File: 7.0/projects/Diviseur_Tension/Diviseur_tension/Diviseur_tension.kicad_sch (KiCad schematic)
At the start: 6 parts, among them Q1 2N2219

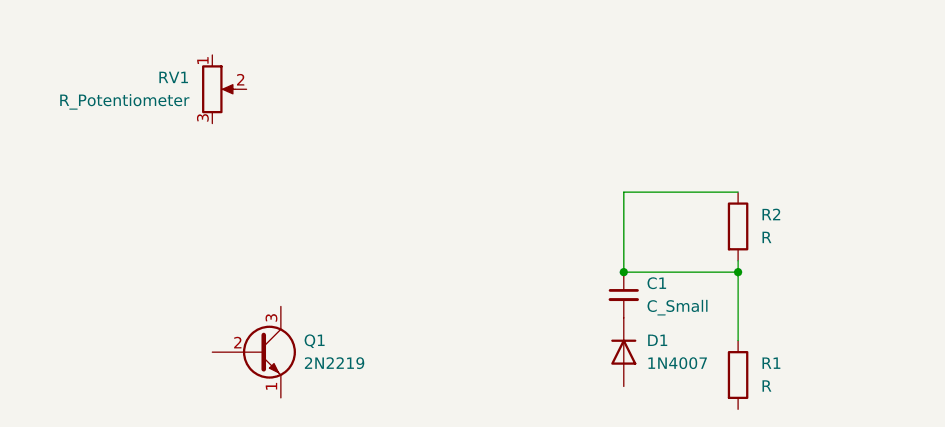
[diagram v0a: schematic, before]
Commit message: new modifcation
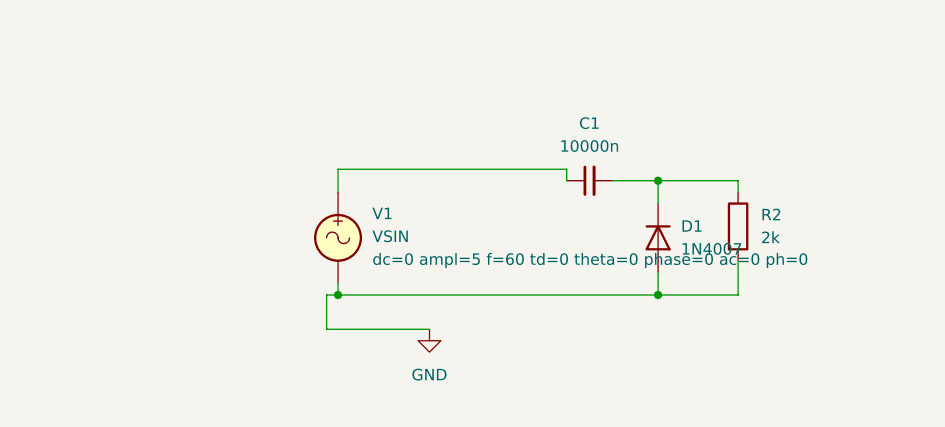
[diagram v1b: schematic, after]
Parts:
- removed Q1: 2N2219, Package_TO_SOT_THT:TO-39-3, symbol Transistor_BJT:2N2219
- removed R1: R, symbol Device:R
- removed RV1: R_Potentiometer, symbol Device:R_Potentiometer
- added V1: VSIN, Connector_PinHeader_2.54mm:PinHeader_1x02_P2.54mm_Vertical, symbol Simulation_SPICE:VSIN
- C1: value C_Small -> 10000n; footprint (none) -> Connector_PinHeader_2.54mm:PinHeader_1x02_P2.54mm_Vertical
- R2: value R -> 2k; footprint (none) -> Resistor_THT:R_Axial_DIN0516_L15.5mm_D5.0mm_P7.62mm_Vertical
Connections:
- net at C1.2, D1.1 (K): now also R2.1
- net GND: now reaches D1.2 (A)
- net GND: now also R2.2, V1.2
- new net: C1.1, V1.1
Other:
- moved on the sheet: C1, D1

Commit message: info
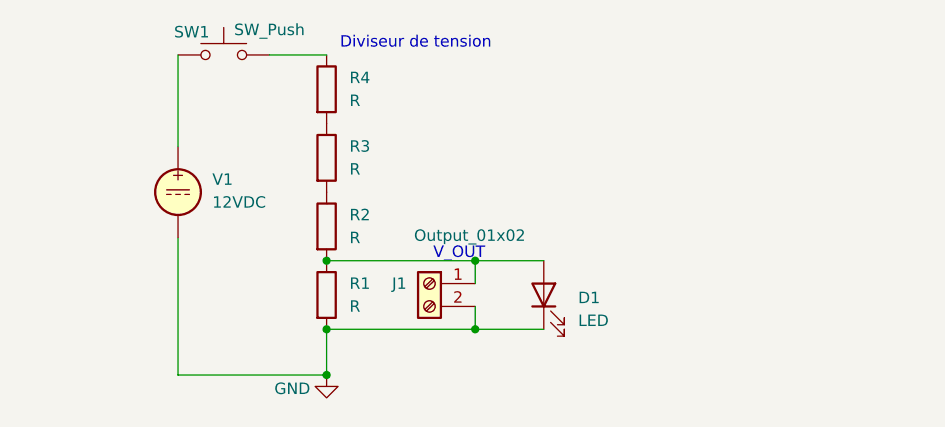
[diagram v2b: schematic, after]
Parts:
- removed C1: 10000n, Connector_PinHeader_2.54mm:PinHeader_1x02_P2.54mm_Vertical, symbol Device:C_Small
- removed D1: 1N4007, Diode_THT:D_DO-41_SOD81_P10.16mm_Horizontal, symbol Diode:1N4007
- removed V1: VSIN, Connector_PinHeader_2.54mm:PinHeader_1x02_P2.54mm_Vertical, symbol Simulation_SPICE:VSIN
- added D1: LED, symbol Device:LED
- added J1: Output_01x02, symbol Connector:Screw_Terminal_01x02
- added R1, R3, R4: R, symbol Device:R
- added SW1: SW_Push, symbol Switch:SW_Push
- added V1: 12VDC, symbol Simulation_SPICE:VDC
- R2: value 2k -> R; footprint Resistor_THT:R_Axial_DIN0516_L15.5mm_D5.0mm_P7.62mm_Vertical -> (none)
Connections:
- net GND: now also D1.1 (K), J1.2 (Pin_2), R1.2, V1.2; no longer R2.2
- net at R2.1: now also R3.2
- new net: D1.2 (A), J1.1 (Pin_1), R1.1, R2.2
- new net: SW1.1, V1.1
- new net: R3.1, R4.2
- new net: R4.1, SW1.2
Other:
- note added: "Diviseur de tension"
- note added: "V_OUT"

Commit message: info info
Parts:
- D1: footprint (none) -> LED_THT:LED_D5.0mm
- J1, V1: footprint (none) -> Connector_PinHeader_2.54mm:PinHeader_1x02_P2.54mm_Vertical
- R1, R2, R3, R4: footprint (none) -> Resistor_THT:R_Axial_DIN0207_L6.3mm_D2.5mm_P10.16mm_Horizontal
- SW1: footprint (none) -> Button_Switch_THT:SW_PUSH_6mm
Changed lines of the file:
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@@
 			)
 		)
-		(property "Footprint" ""
+		(property "Footprint" "Resistor_THT:R_Axial_DIN0207_L6.3mm_D2.5mm_P10.16mm_Horizontal"
 			(at 140.462 95.25 90)
 			(effects
@@
 			)
 		)
-		(property "Footprint" ""
+		(property "Footprint" "Connector_PinHeader_2.54mm:PinHeader_1x02_P2.54mm_Vertical"
 			(at 125.73 83.82 0)
 			(effects
@@
 			)
 		)
-		(property "Footprint" ""
+		(property "Footprint" "Resistor_THT:R_Axial_DIN0207_L6.3mm_D2.5mm_P10.16mm_Horizontal"
 			(at 140.462 80.01 90)
 			(effects
@@
 			)
 		)
-		(property "Footprint" ""
+		(property "Footprint" "Resistor_THT:R_Axial_DIN0207_L6.3mm_D2.5mm_P10.16mm_Horizontal"
 			(at 140.462 87.63 90)
 			(effects
@@
 			)
 		)
-		(property "Footprint" ""
+		(property "Footprint" "LED_THT:LED_D5.0mm"
 			(at 166.37 95.25 0)
 			(effects
@@
 			)
 		)
-		(property "Footprint" ""
+		(property "Footprint" "Resistor_THT:R_Axial_DIN0207_L6.3mm_D2.5mm_P10.16mm_Horizontal"
 			(at 140.462 72.39 90)
 			(effects
@@
 			)
 		)
-		(property "Footprint" ""
+		(property "Footprint" "Connector_PinHeader_2.54mm:PinHeader_1x02_P2.54mm_Vertical"
 			(at 153.67 93.98 0)
 			(effects
@@
 			)
 		)
-		(property "Footprint" ""
+		(property "Footprint" "Button_Switch_THT:SW_PUSH_6mm"
 			(at 130.81 63.5 0)
 			(effects
